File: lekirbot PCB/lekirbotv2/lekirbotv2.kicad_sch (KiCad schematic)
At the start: 56 parts, among them IC3 7404D, J1 455-1750-1-ND, J2 455-1750-1-ND, J3 Conn_01x04_Pin, M1A0 CONN_01, M1B0 CONN_01, M2A0 CONN_01, M2B0 CONN_01, SW1 SW_Push, U1 TB6612FNG, U2 QRE11131{colon}1, U5 QRE11131{colon}1, U6 QRE11131{colon}1, U7 QRE11131{colon}1, U8 QRE11131{colon}1

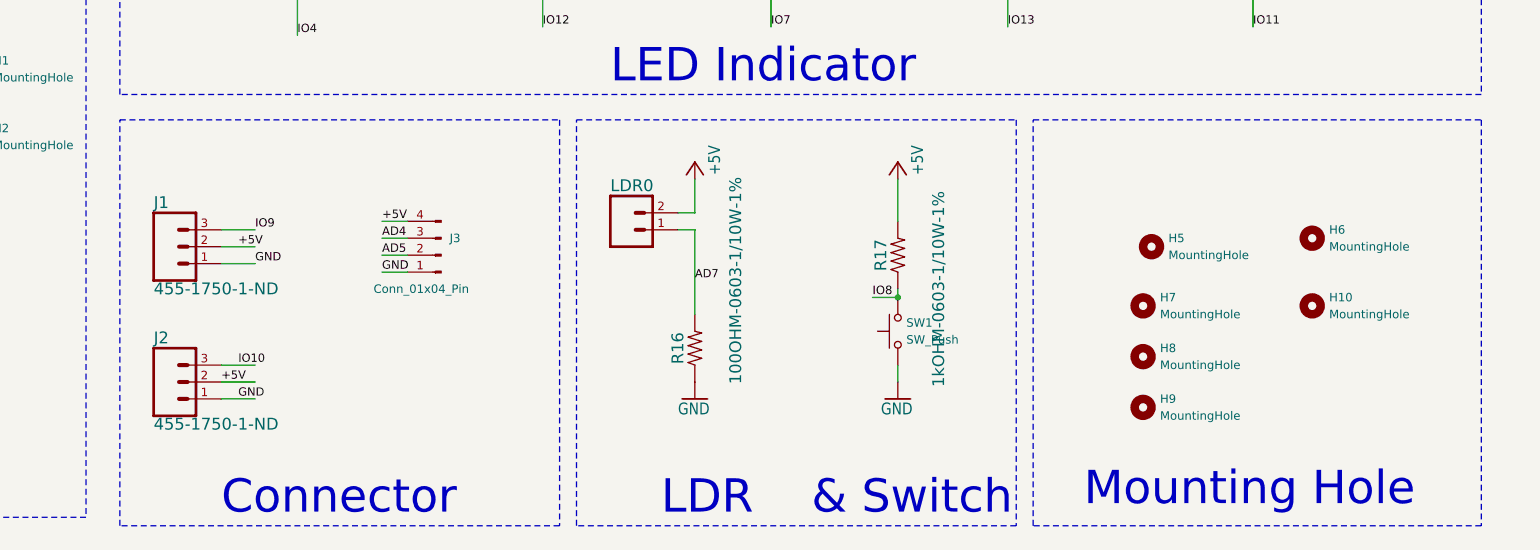
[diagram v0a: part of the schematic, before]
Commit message: Updated lekirbotv2
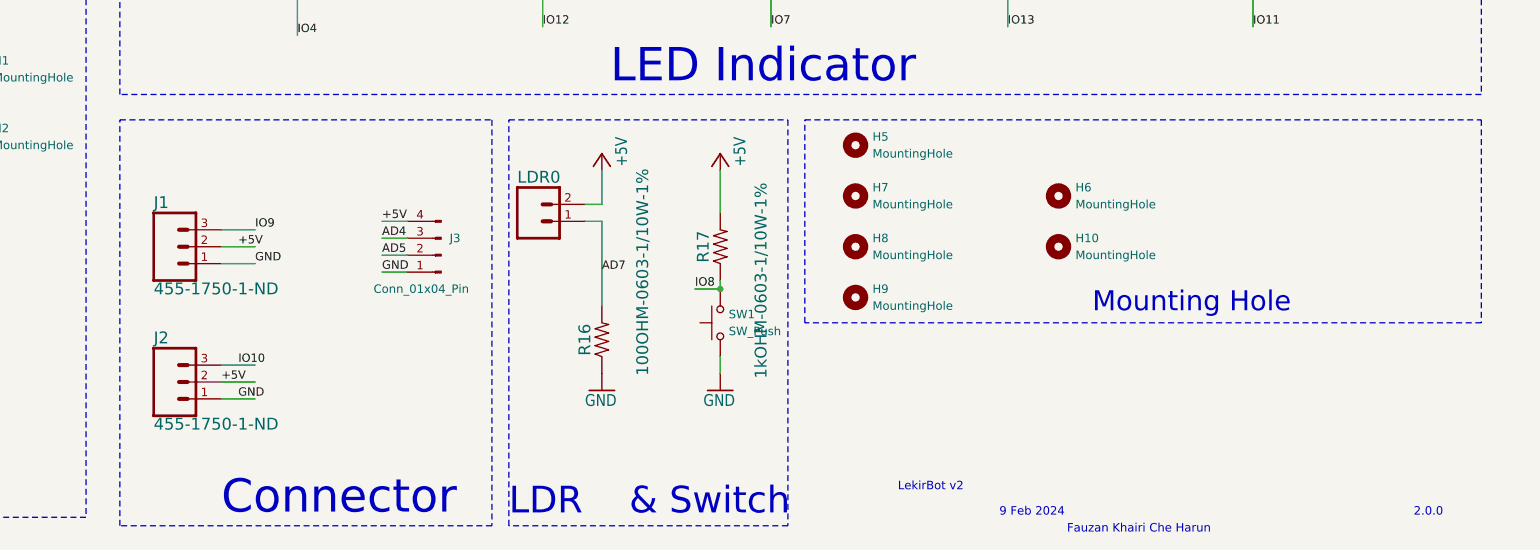
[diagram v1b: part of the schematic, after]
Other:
- note added: "2.0.0"
- note added: "9 Feb 2024"
- note added: "Fauzan Khairi Che Harun"
- note added: "LekirBot v2"
- moved on the sheet: H10, H5, H6, H7, H8, H9, LDR0, R16, R17, SW1
